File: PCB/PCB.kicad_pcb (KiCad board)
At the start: 2 copper layers, 61.9 x 63.1 mm, 15 parts, among them M1 Motor_Servo, M2 Motor_Servo, SW1 RotaryEncoder_Switch, SW2 RotaryEncoder_Switch, SW3 SW_Push, SW4 SW_Push, SW5 SW_Push, SW6 SW_Push, U1 XIAO-RP2040-DIP

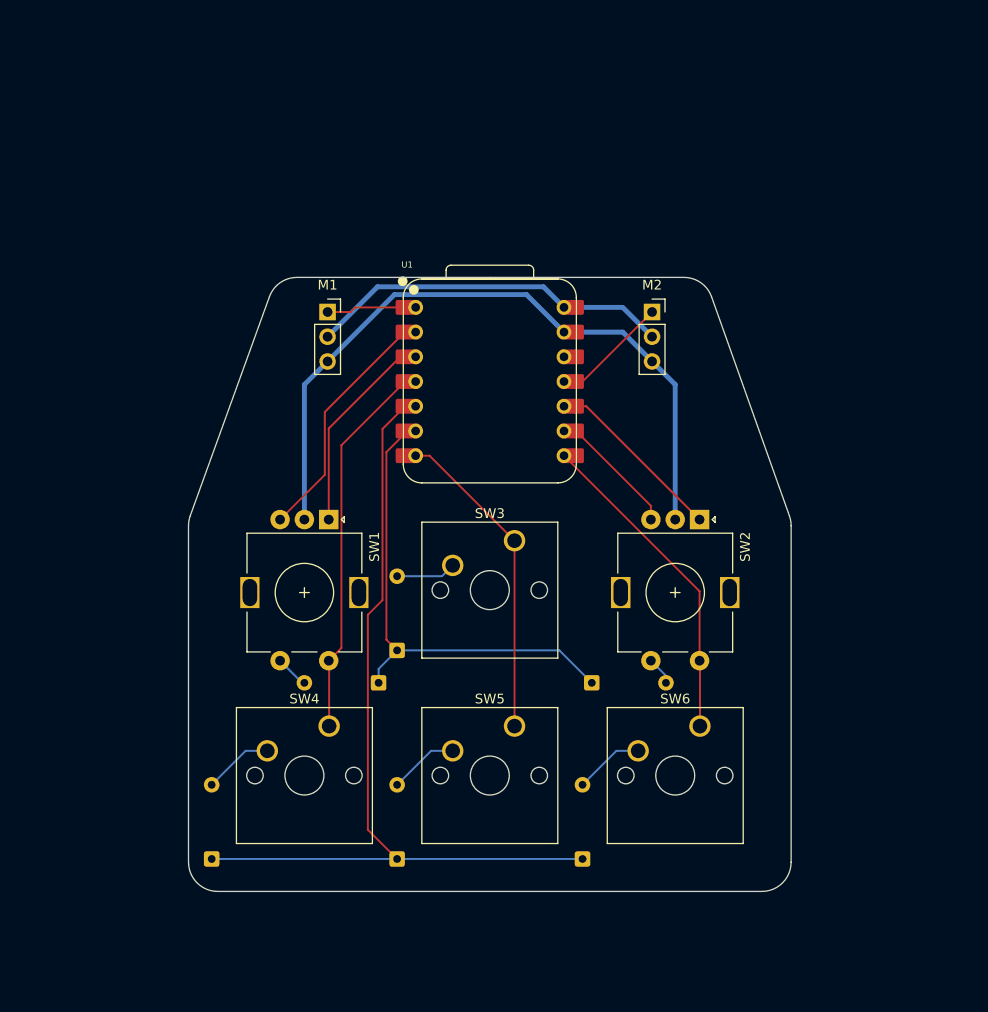
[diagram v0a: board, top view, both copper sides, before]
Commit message: bleh
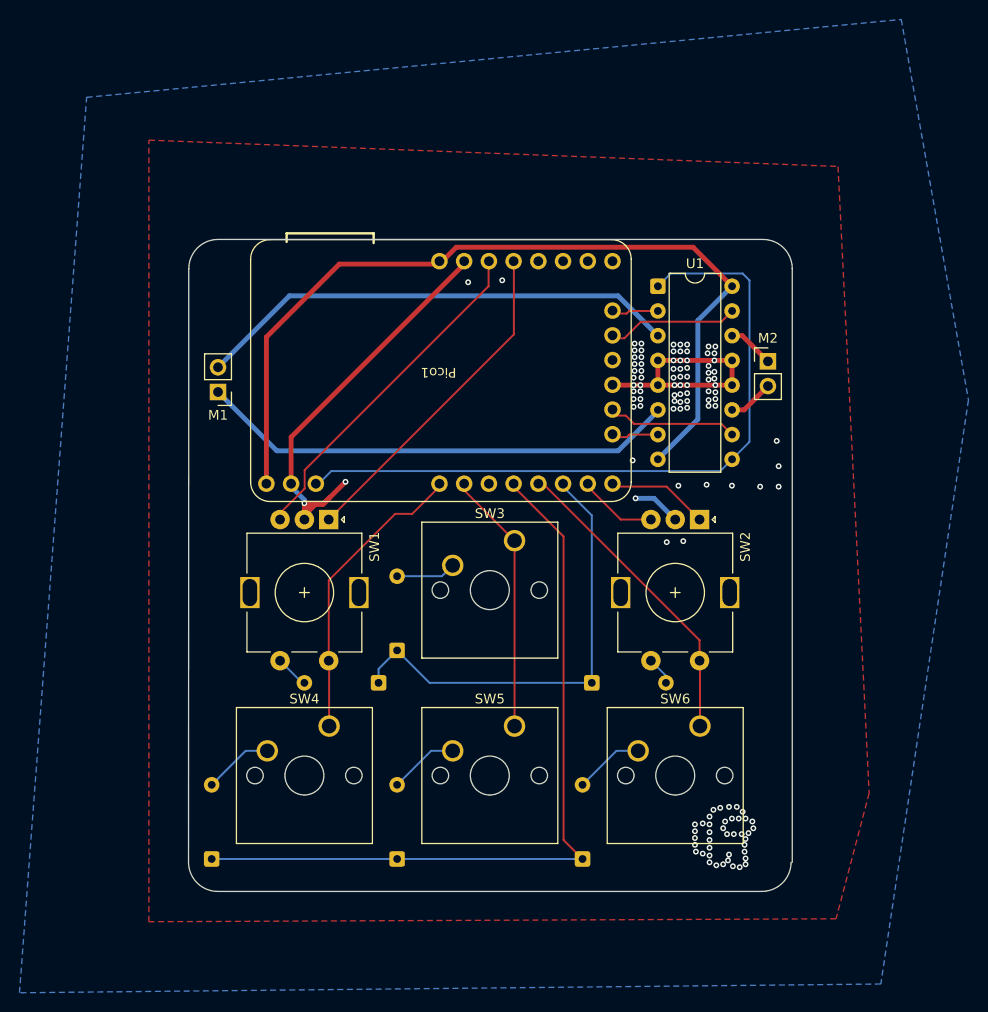
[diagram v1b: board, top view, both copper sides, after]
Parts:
- added Pico1: ~, Taranium-libs:Taranium_Pico, F.Cu at (156.8, 75.3)
- M1, M2: value Motor_Servo -> Conn_01x02_Pin; footprint Connector_PinSocket_2.54mm:PinSocket_1x03_P2.54mm_Vertical -> Connector_PinHeader_2.54mm:PinHeader_1x02_P2.54mm_Vertical
- U1: value XIAO-RP2040-DIP -> L293D; footprint Taranium-libs:XIAO-RP2040-DIP -> Package_DIP:DIP-16_W7.62mm
- moved U1 19.9 mm to (179.2, 66.4)
- moved M1 13.9 mm to (134.0, 77.3), turned to 180 degrees
- moved M2 12.9 mm to (190.5, 74.1)
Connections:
- M1 pad 1: S1 -> M1 P2
- M1 pad 2: +5V -> M1 P1
- M2 pad 1: S2 -> M2 P2
- M2 pad 2: +5V -> M2 P1
- U1 pad 1: S1 -> +3V3
- U1 pad 10: A2 -> 3A
- U1 pad 11: S2 -> M2 P1
- U1 pad 12: +3V3 -> GND
- U1 pad 14: +5V -> M2 P2
- U1 pad 2: B1 -> 1A
- U1 pad 3: A1 -> M1 P1
- U1 pad 4: C1 -> GND
- U1 pad 5: R2 -> GND
- U1 pad 6: R1 -> M1 P2
- U1 pad 7: C2 -> 2A
- U1 pad 8: C3 -> +5V
- U1 pad 9: B2 -> +3V3
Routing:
- net +3V3: track 0.00 -> 73.3 mm
- net +5V: track 37.6 -> 89.6 mm
- net M1 P1: track 0.00 -> 49.9 mm
- net M1 P2: track 0.00 -> 49.5 mm
- net A1: track 20.5 -> 34.1 mm
- net 4A: track 0.00 -> 13.4 mm
- net 3A: track 0.00 -> 13.2 mm
- net S2: track 12.0 -> 0.00 mm
- net B1: track 25.7 -> 35.4 mm
- net C1: track 39.7 -> 30.4 mm
- net S1: track 9.25 -> 0.00 mm
- net R2: track 88.5 -> 79.3 mm
- net A2: track 18.8 -> 10.3 mm
- net C2: track 32.8 -> 26.7 mm
- net B2: track 13.5 -> 7.89 mm
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- added copper zone on B.Cu, net GND
- added copper zone on F.Cu, net GND
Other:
- board size 61.9 x 63.1 mm -> 62 x 67 mm
